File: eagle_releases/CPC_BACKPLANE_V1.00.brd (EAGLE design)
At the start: 99.6 x 81.3 mm, 11 parts

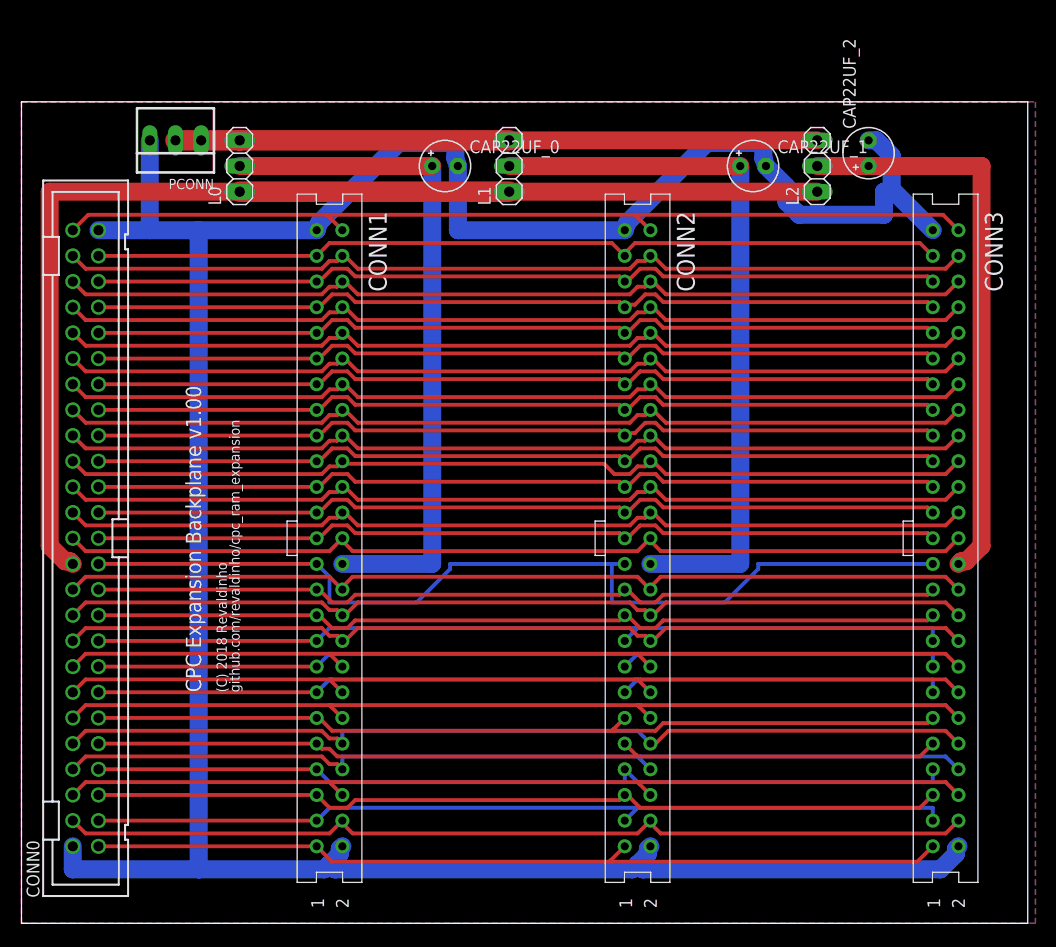
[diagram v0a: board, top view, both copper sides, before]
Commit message: Update cpc_backplane PCB
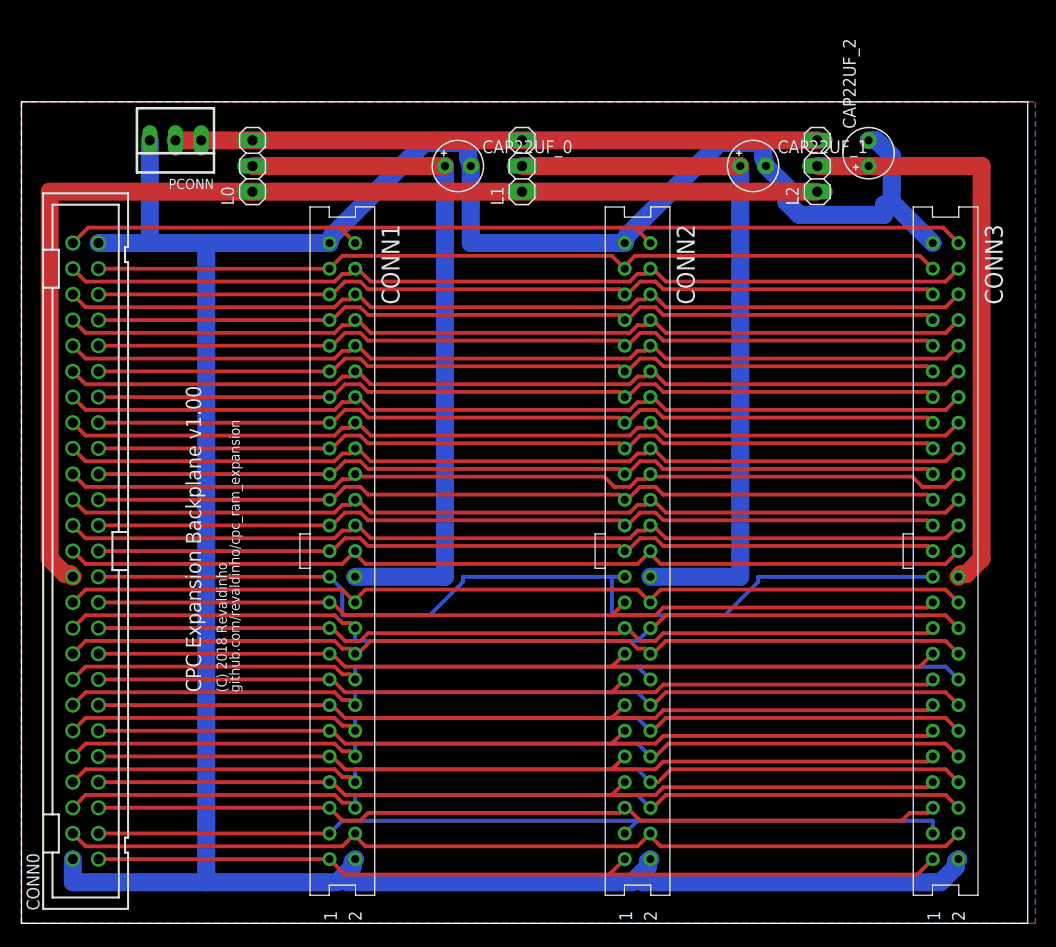
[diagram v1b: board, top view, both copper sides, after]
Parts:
- moved CONN1 1.80 mm to (31.8, 36.8)
- moved CAP22UF_0 1.27 mm to (43.2, 74.9)
- moved CONN0 1.27 mm to (6.35, 36.8)
- moved CONN2 1.27 mm to (61.0, 36.8)
- moved CONN3 1.27 mm to (91.4, 36.8)
- moved L1 1.27 mm to (49.5, 74.9)
- moved L0 1.27 mm to (22.9, 74.9)
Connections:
- net VDD renamed VDD1
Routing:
- net VSS: track 282.5 -> 286.1 mm
- net VDD_CPC: track 114.0 -> 115.3 mm
- net VDD3: track 56.9 -> 58.1 mm
- net VDD1: track 67.3 -> 68.6 mm
- net RAMRD_B: track 86.1 -> 85.3 mm
- net NMI_B: track 86.1 -> 85.3 mm
- net BUSACK_B: track 86.1 -> 85.3 mm
- net HALT_B: track 86.1 -> 85.3 mm
- net ROMDIS: track 92.2 -> 91.5 mm
- net READY: track 92.1 -> 91.5 mm
- net RAMDIS: track 92.1 -> 91.5 mm
- net BUSRQ_B: track 92.1 -> 91.5 mm
- net RFSH_B: track 84.8 -> 85.3 mm
